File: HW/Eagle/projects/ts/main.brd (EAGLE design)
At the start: 95 x 48 mm, 24 parts, among them IC1 4050D, U1 ATMEGA328P-PU, U2 LM2576T, U3 LE33CZ

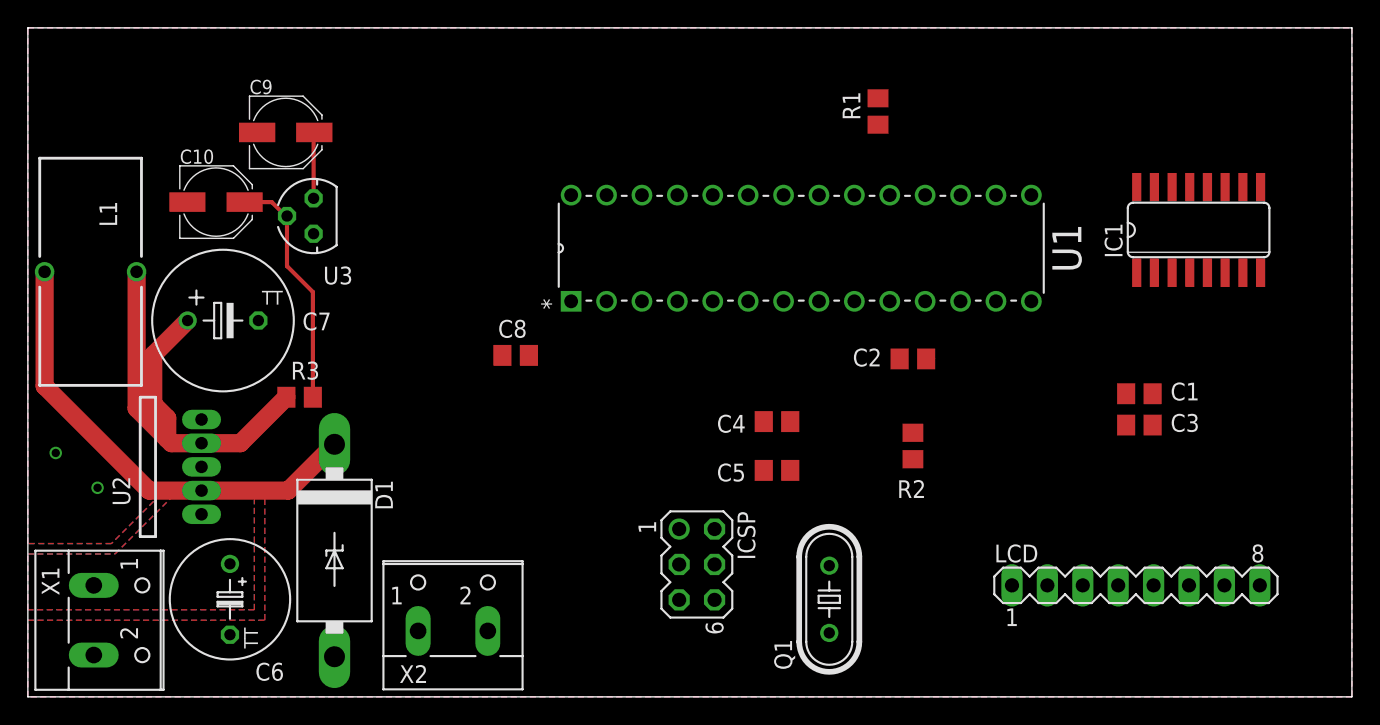
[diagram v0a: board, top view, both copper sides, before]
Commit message: Many changes
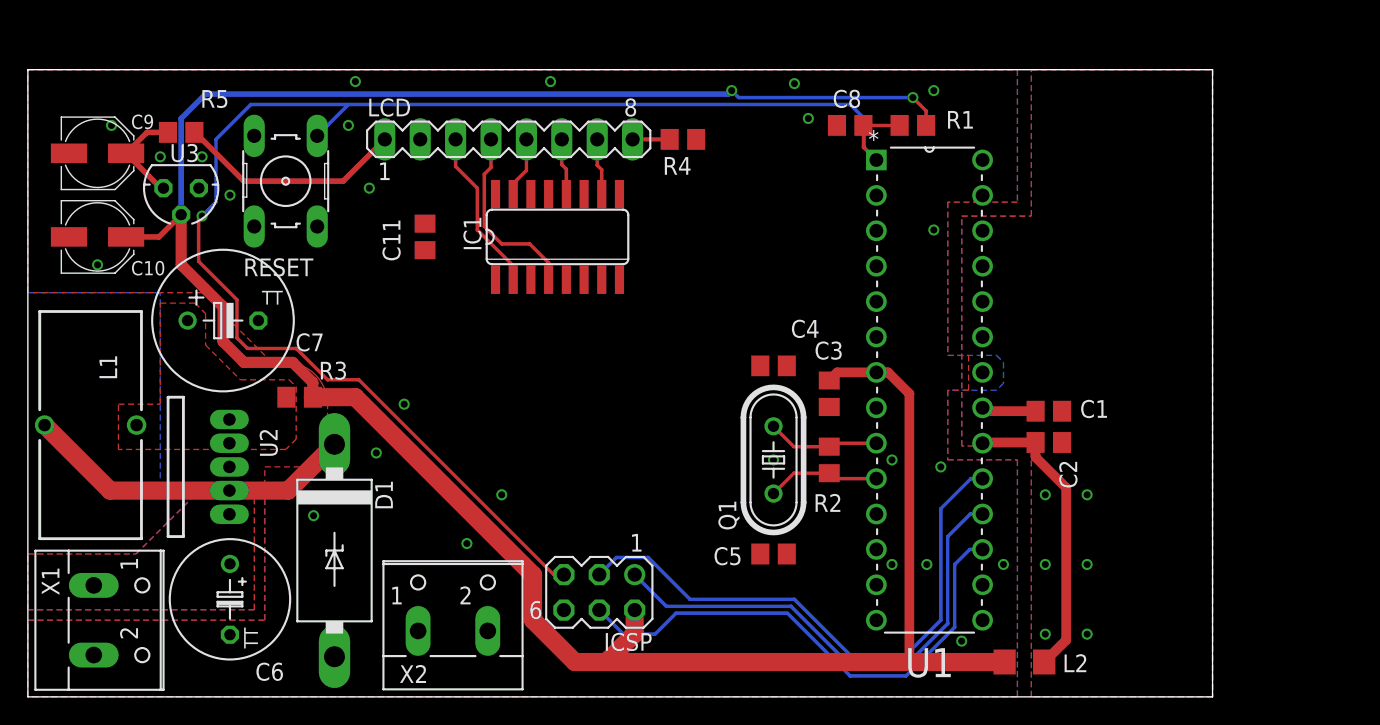
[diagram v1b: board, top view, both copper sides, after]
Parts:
- added C11: 100nF, rcl:C0805
- added L2: 10uH, misc:L1206
- added R4: 330R, rcl:R0805
- added R5: 0R, rcl:R0805
- added RESET: (no value), switch-omron:B3F-10XX
- R3: value 0 -> 0R
- U3: value LE33CZ -> HT7533
- moved LCD 55.2 mm to (34.5, 40.0)
- moved IC1 46.0 mm to (38.0, 33.0)
- moved U1 30.7 mm to (68.5, 5.50), turned to 0 degrees
- moved C8 29.1 mm to (59.0, 41.0)
- moved C3 22.4 mm to (57.5, 21.8), turned to 90 degrees
- moved C9 13.6 mm to (5.00, 39.0)
- moved C2 11.4 mm to (73.2, 18.2), turned to 180 degrees
- moved L1 11.0 mm to (4.50, 19.5)
- moved Q1 10.8 mm to (53.5, 17.0)
- moved U3 9.71 mm to (11.0, 36.5), turned to 180 degrees
- moved C10 8.86 mm to (5.00, 33.0)
- moved ICSP 7.28 mm to (41.0, 7.50), turned to 180 degrees
- moved C1 6.62 mm to (73.2, 20.5)
- moved R2 6.08 mm to (57.5, 17.0)
- moved C5 6.01 mm to (53.5, 10.2)
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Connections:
- net N$1 renamed AREF
- net N$2 renamed MISO
- removed net N$5: ICSP.3, U1.19
- removed net N$6: ICSP.4, U1.17
- new net AVCC: C2.2, L2.1, U1.20
- new net LCD_DC: IC1.15, LCD.5
- new net LCD_LED: LCD.8, R4.2
- new net LCD_MOSI: IC1.12, LCD.6
- new net LCD_RST: IC1.4, LCD.4
- new net LCD_SCE: IC1.2, LCD.3
- new net LCD_SCK: IC1.10, LCD.7
- new net MOSI: IC1.11, ICSP.4, U1.17
- new net N$1: C9.+, R5.2, U3.3
- new net N$2: R4.1
- new net RXD: U1.2
- new net SCK: IC1.9, ICSP.3, U1.19
- new net TXD: U1.3
- net +3V3: now also C11.2, R5.1; no longer C9.+, U3.3
- net GND: now also C11.1, IC1.7, RESET.3
- net NRST: now also RESET.1
- net VCC: now also L2.2; no longer C2.2, U1.20
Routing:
- net VCC: track 17.8 -> 176.4 mm, vias 0 -> 2
- net NRST: track 0.00 -> 106.3 mm, vias 0 -> 1
- net SCK: track 0.00 -> 41.3 mm
- net MOSI: track 0.00 -> 37.1 mm
- net MISO: track 0.00 -> 36.0 mm
- net N$8: track 32.9 -> 0.00 mm
- net AVCC: track 0.00 -> 21.1 mm
- net LCD_RST: track 0.00 -> 13.4 mm
- net LCD_SCE: track 0.00 -> 11.8 mm
- net +3V3: track 4.75 -> 16.4 mm
- net N$7: track 33.5 -> 24.1 mm
- net N$3: track 0.00 -> 8.15 mm
- net N$4: track 0.00 -> 8.09 mm
- net N$1: track 0.00 -> 7.34 mm
- net LCD_DC: track 0.00 -> 4.32 mm
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- added copper zone on layer 1, net N$8
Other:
- board size 95 x 48 mm -> 85 x 45 mm
